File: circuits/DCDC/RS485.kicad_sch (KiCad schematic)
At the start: 44 parts, among them J1 Conn_01x07_MountingPin, Q1 S8550, Q2 S8550, Q3 S8550, Q4 S8550, Q5 S8550, Q6 S8550, U1 MAX3485, U2 MAX3485, U3 MAX3485, U4 MAX3485, U5 MAX3485, U6 MAX3485

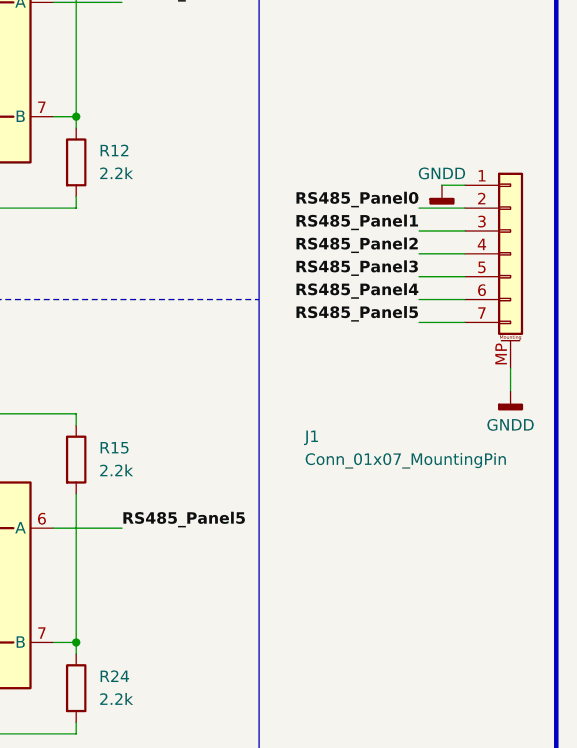
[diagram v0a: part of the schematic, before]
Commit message: raspi基板回路図
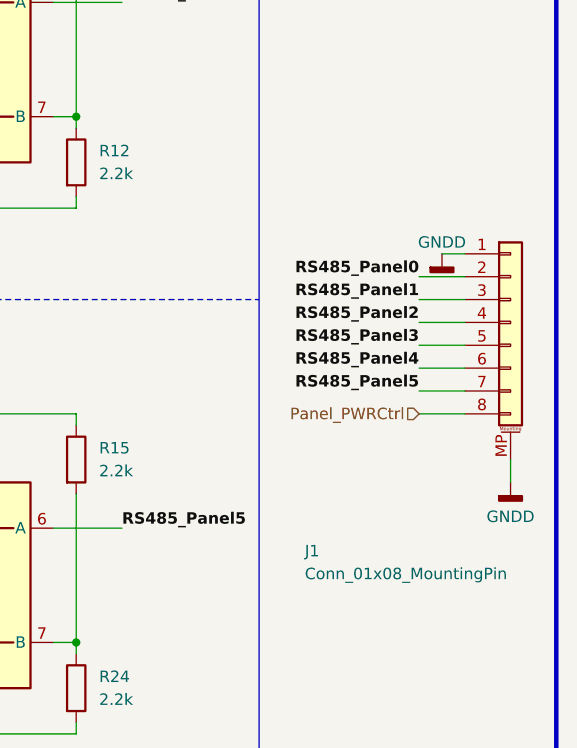
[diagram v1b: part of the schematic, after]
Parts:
- removed J1: Conn_01x07_MountingPin, Connector_Molex:Molex_PicoBlade_53261-0771_1x07-1MP_P1.25mm_Horizontal, symbol Connector_Generic_MountingPin:Conn_01x07_MountingPin
- added J1: Conn_01x08_MountingPin, Connector_Molex:Molex_PicoBlade_53261-0871_1x08-1MP_P1.25mm_Horizontal, symbol Connector_Generic_MountingPin:Conn_01x08_MountingPin
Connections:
- net GNDD: now also J1.1 (Pin_1), J1.MP (MountPin)
- net RS485_Panel0: now also J1.2 (Pin_2)
- net RS485_Panel1: now also J1.3 (Pin_3)
- net RS485_Panel2: now also J1.4 (Pin_4)
- net RS485_Panel3: now also J1.5 (Pin_5)
- net RS485_Panel4: now also J1.6 (Pin_6)
- net RS485_Panel5: now also J1.7 (Pin_7)
- new net Panel_PWRCtrl: J1.8 (Pin_8)

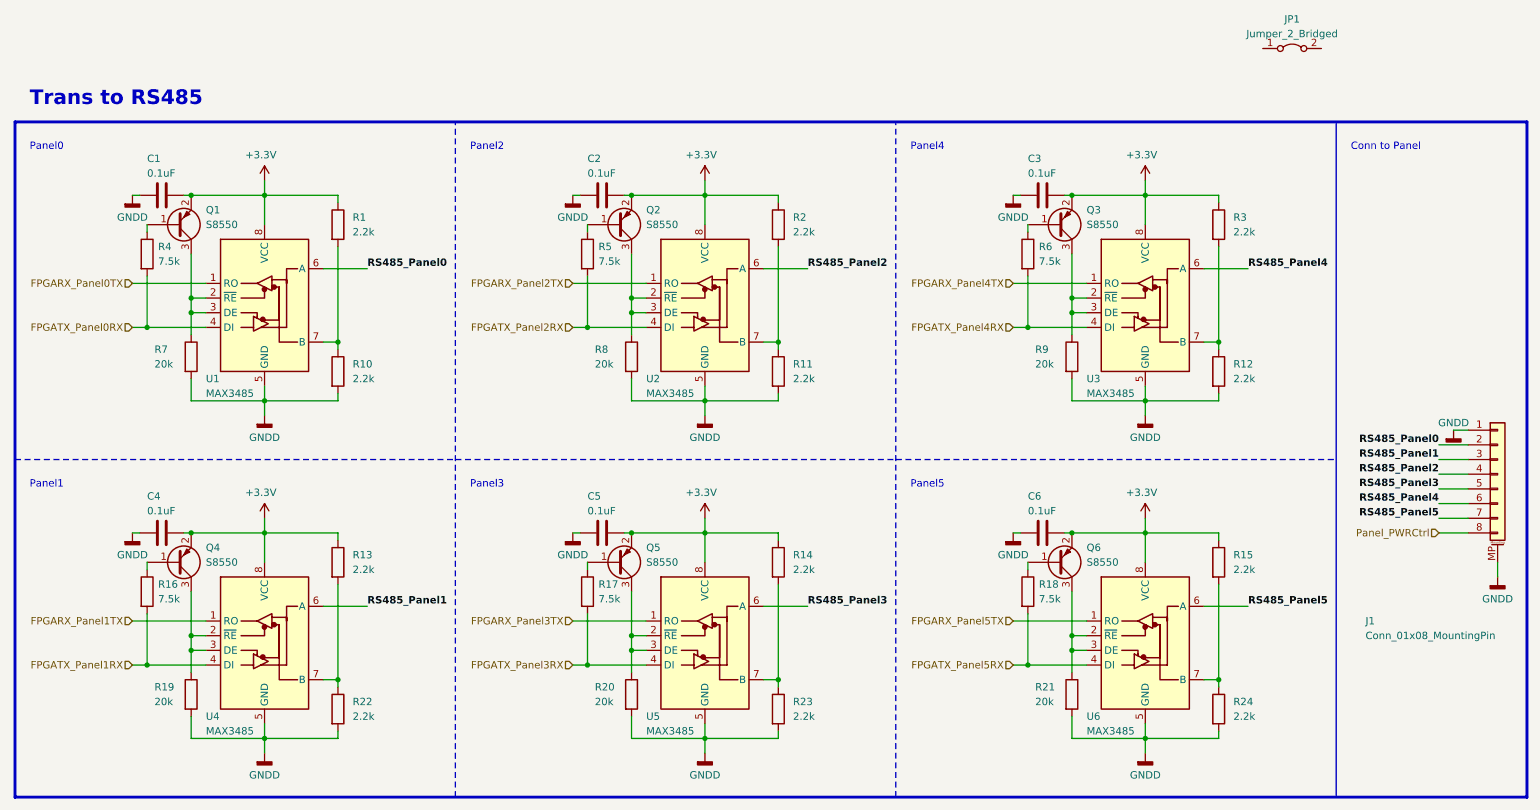
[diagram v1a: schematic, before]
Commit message: 発注第3弾
DCDC、MD追加
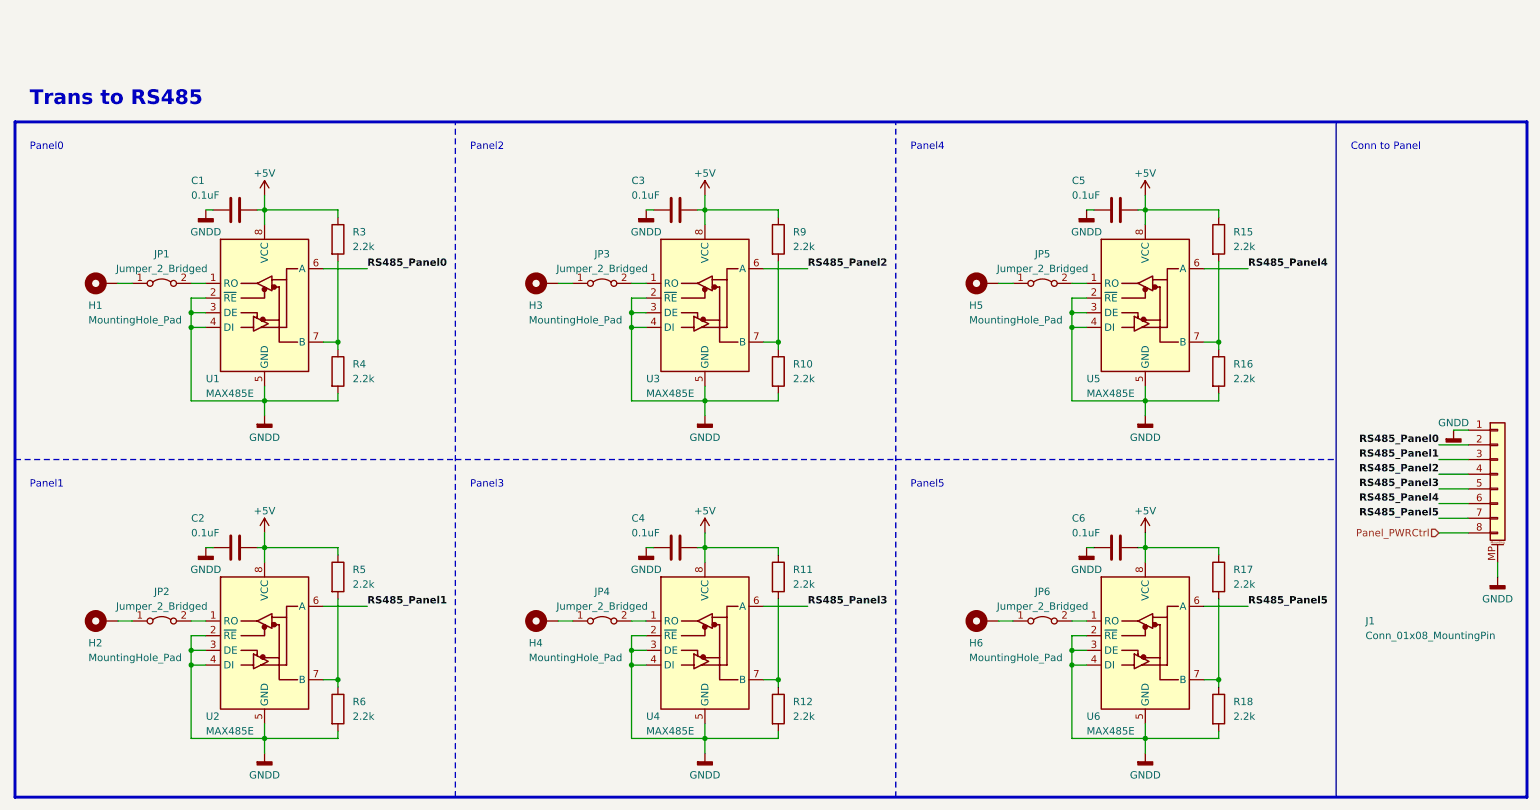
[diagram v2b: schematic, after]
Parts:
- removed Q1, Q2, Q3, Q4, Q5, Q6: S8550, Package_TO_SOT_SMD:SOT-23, symbol Device:Q_PNP_BEC
- removed R1, R13, R14, R2, R22, R23, R24: 2.2k, Resistor_SMD:R_0402_1005Metric, symbol Device:R
- removed R19, R20, R21, R7, R8: 20k, Resistor_SMD:R_0402_1005Metric, symbol Device:R
- removed U1, U2, U3, U4, U5, U6: MAX3485, Package_SO:SOP-8_3.9x4.9mm_P1.27mm, symbol Interface_UART:MAX3485
- added H1, H2, H3, H4, H5, H6: MountingHole_Pad, MountingHole:MountingHole_2.2mm_M2_Pad, symbol Mechanical:MountingHole_Pad
- added JP2, JP3, JP4, JP5, JP6: Jumper_2_Bridged, Jumper:SolderJumper-2_P1.3mm_Bridged_RoundedPad1.0x1.5mm, symbol Jumper:Jumper_2_Bridged
- added U1, U2, U3, U4, U5, U6: MAX485E, Package_SO:SOP-8_3.9x4.9mm_P1.27mm, symbol Interface_UART:MAX485E
- R16, R17, R18, R4, R5, R6: value 7.5k -> 2.2k; footprint Resistor_SMD:R_0603_1608Metric -> Resistor_SMD:R_0402_1005Metric
- R9: value 20k -> 2.2k
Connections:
- net +3.3V is gone; now on net +5V: C1.1, C2.1, C3.1, C4.1, C5.1, C6.1, R15.1, R3.1
- net FPGATX_Panel0RX is gone; now on net GNDD: R4.2
- net FPGATX_Panel1RX is gone; now on net GNDD: R16.2
- net FPGATX_Panel2RX is gone; now on an unnamed net: R5.2
- net FPGATX_Panel3RX is gone; now on an unnamed net: R17.2
- net FPGATX_Panel4RX is gone; now on net GNDD: R6.2
- net FPGATX_Panel5RX is gone; now on net GNDD: R18.2
- net GNDD: now also U1.2 (~{RE}), U1.3 (DE), U1.4 (DI), U1.5 (GND), U2.2 (~{RE}), U2.3 (DE), U2.4 (DI), U2.5 (GND), U3.2 (~{RE}), U3.3 (DE), U3.4 (DI), U3.5 (GND), U4.2 (~{RE}), U4.3 (DE), U4.4 (DI), U4.5 (GND), U5.2 (~{RE}), U5.3 (DE), U5.4 (DI), U5.5 (GND), U6.2 (~{RE}), U6.3 (DE), U6.4 (DI), U6.5 (GND); no longer R11.2, R9.2
- net RS485_Panel0: now also U1.6 (A)
- net RS485_Panel1: now also U2.6 (A)
- net RS485_Panel2: now also U3.6 (A)
- net RS485_Panel3: now also U4.6 (A)
- net RS485_Panel4: now also U5.6 (A)
- net RS485_Panel5: now also U6.6 (A)
- net +5V: now reaches R5.1
- net +5V: now also R11.1, R17.1, R9.1, U1.8 (VCC), U2.8 (VCC), U3.8 (VCC), U4.8 (VCC), U5.8 (VCC), U6.8 (VCC)
- net at R12.1: now also R11.2, U4.7 (B); no longer R3.2
- net at R16.1: now also R15.2, U5.7 (B)
- net at R10.1: now also R9.2, U3.7 (B)
- net at R18.1: now also U6.7 (B)
- net at R4.1: now also R3.2, U1.7 (B)
- net at JP1.1 (A): now also H1.1
- net at JP1.2 (B): now also U1.1 (RO)
- net at R6.1: now also U2.7 (B)
- new net: H4.1, JP4.1 (A)
- new net: H5.1, JP5.1 (A)
- new net: JP5.2 (B), U5.1 (RO)
- new net: JP4.2 (B), U4.1 (RO)
- new net: H3.1, JP3.1 (A)
- new net: JP3.2 (B), U3.1 (RO)
- new net: H2.1, JP2.1 (A)
- new net: JP2.2 (B), U2.1 (RO)
- new net: H6.1, JP6.1 (A)
- new net: JP6.2 (B), U6.1 (RO)
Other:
- moved on the sheet: JP1
